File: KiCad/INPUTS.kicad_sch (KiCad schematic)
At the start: 16 parts

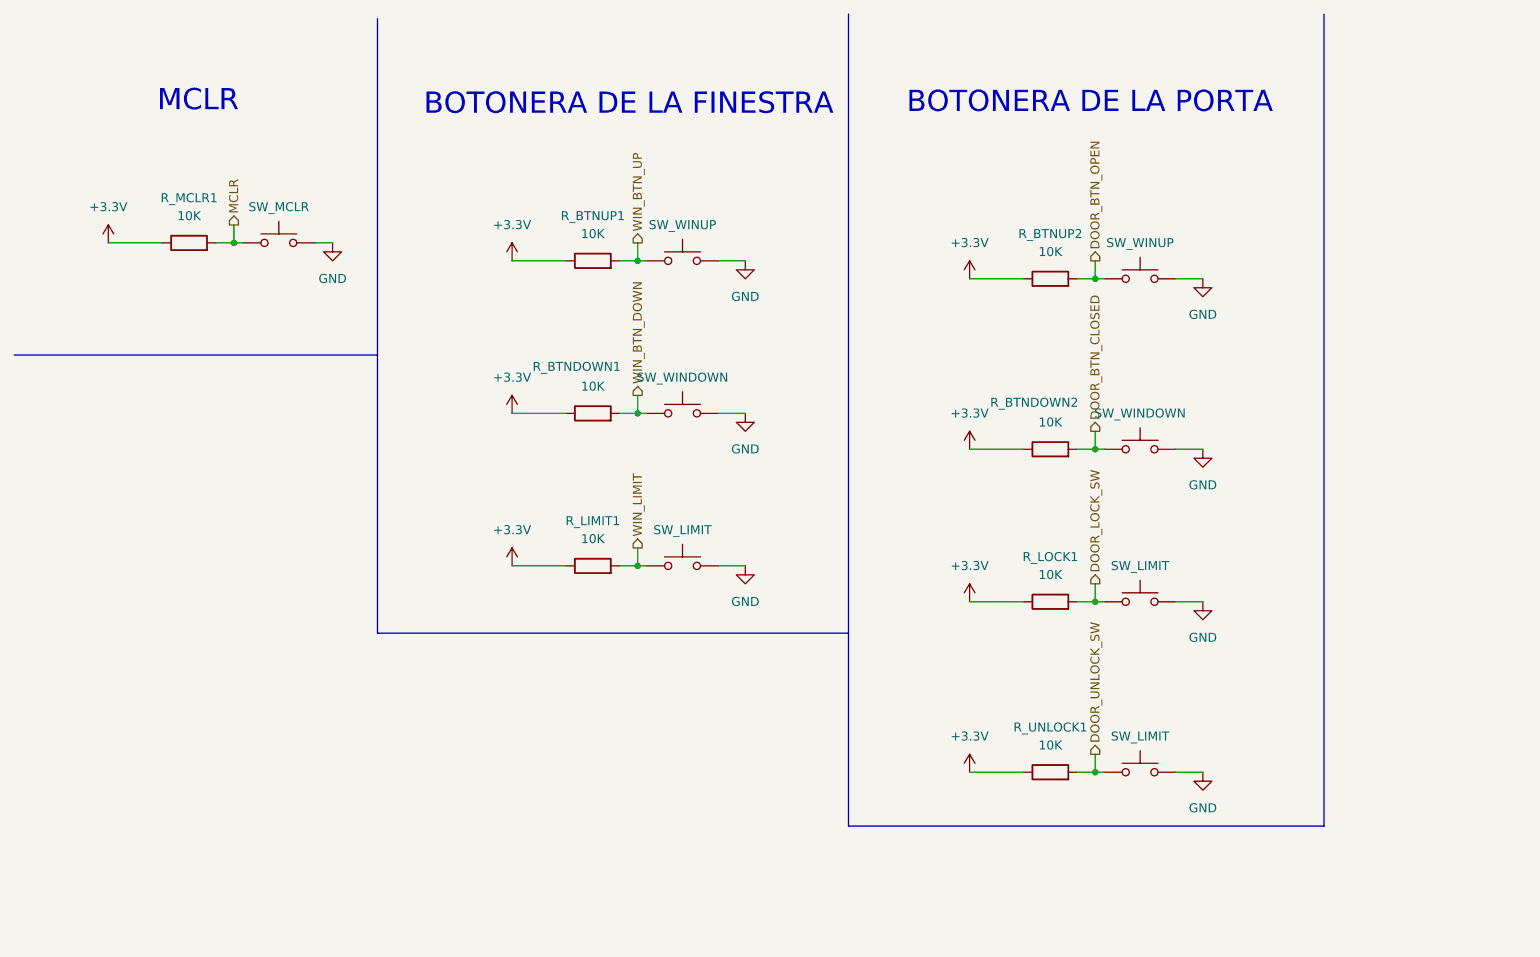
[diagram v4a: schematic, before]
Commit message: Inputs
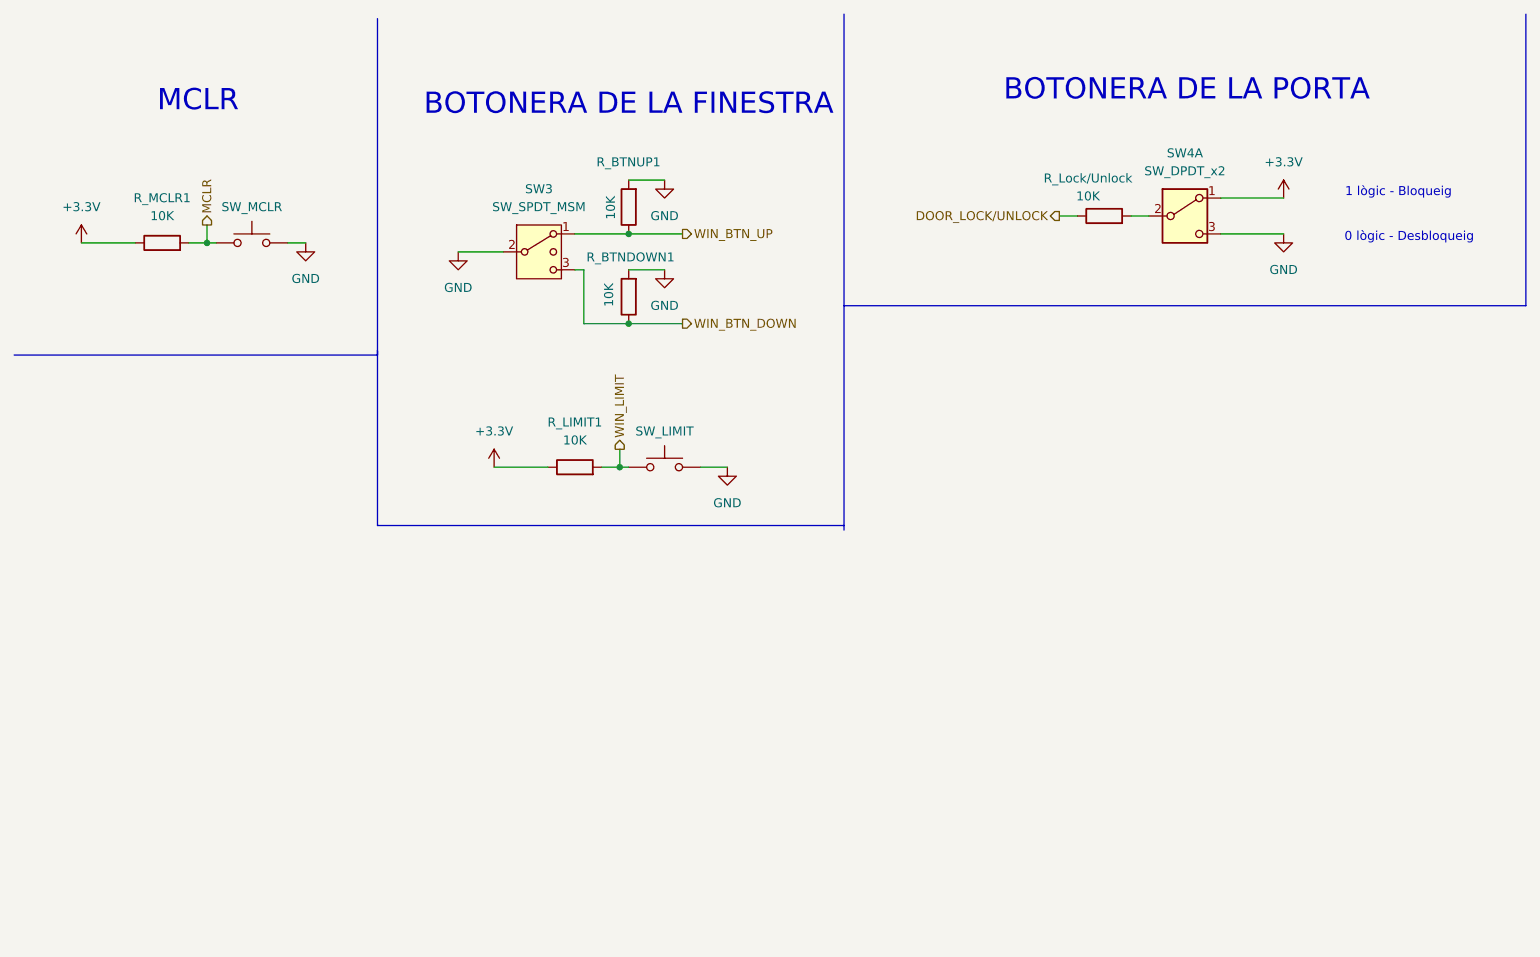
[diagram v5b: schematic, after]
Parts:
- removed R_BTNDOWN2, R_BTNUP2, R_LOCK1: 10K, Resistor_SMD:R_0805_2012Metric, symbol Device:R
- removed SW_UP2, SW_UP5: SW_WINUP, Button_Switch_SMD:SW_SPST_TL3342, symbol Switch:SW_Push
- removed SW_UP3, SW_UP6: SW_WINDOWN, Button_Switch_SMD:SW_SPST_TL3342, symbol Switch:SW_Push
- removed SW_UP7, SW_UP8: SW_LIMIT, Button_Switch_SMD:SW_SPST_TL3342, symbol Switch:SW_Push
- added SW3: SW_SPDT_MSM, Button_Switch_SMD:SW_DPDT_CK_JS202011JCQN, symbol Switch:SW_SPDT_MSM
- added SW4: SW_DPDT_x2, Button_Switch_THT:SW_CK_JS202011CQN_DPDT_Straight, symbol Switch:SW_DPDT_x2
- renumbered R_UNLOCK1 to R_Lock/Unlock
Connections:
- net +3.3V: now also SW4.1 (A); no longer R_BTNDOWN1.1, R_BTNUP1.1, R_Lock/Unlock.1
- net GND: now also R_BTNDOWN1.2, R_BTNUP1.2, SW3.2 (3), SW4.3 (C)
- net WIN_BTN_DOWN: now also R_BTNDOWN1.1, SW3.3 (4); no longer R_BTNDOWN1.2
- net WIN_BTN_UP: now also R_BTNUP1.1, SW3.1; no longer R_BTNUP1.2
- net DOOR_UNLOCK_SW: no longer names the net of R_Lock/Unlock.2
- net DOOR_UNLOCK_SW: now also SW4.2 (B)
- new net DOOR_LOCK/UNLOCK: R_Lock/Unlock.1
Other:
- note added: "0 lògic - Desbloqueig"
- note added: "1 lògic - Bloqueig"
- moved on the sheet: R_BTNDOWN1, R_BTNUP1, R_LIMIT1, R_Lock/Unlock, R_MCLR1
